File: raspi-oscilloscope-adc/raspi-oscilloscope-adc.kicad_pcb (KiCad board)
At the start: 2 copper layers, 80 x 47.5 mm, 26 parts, among them J1 Conn_Coaxial, J2 Conn_01x10_Male, J3 Conn_01x02_Male, SW1 SR10010F-0106-20F0B-C7-N-0027, U1 ECS-220B-100, U2 TLC5510INSR, U3 OPA690, U4 SN74LS245N

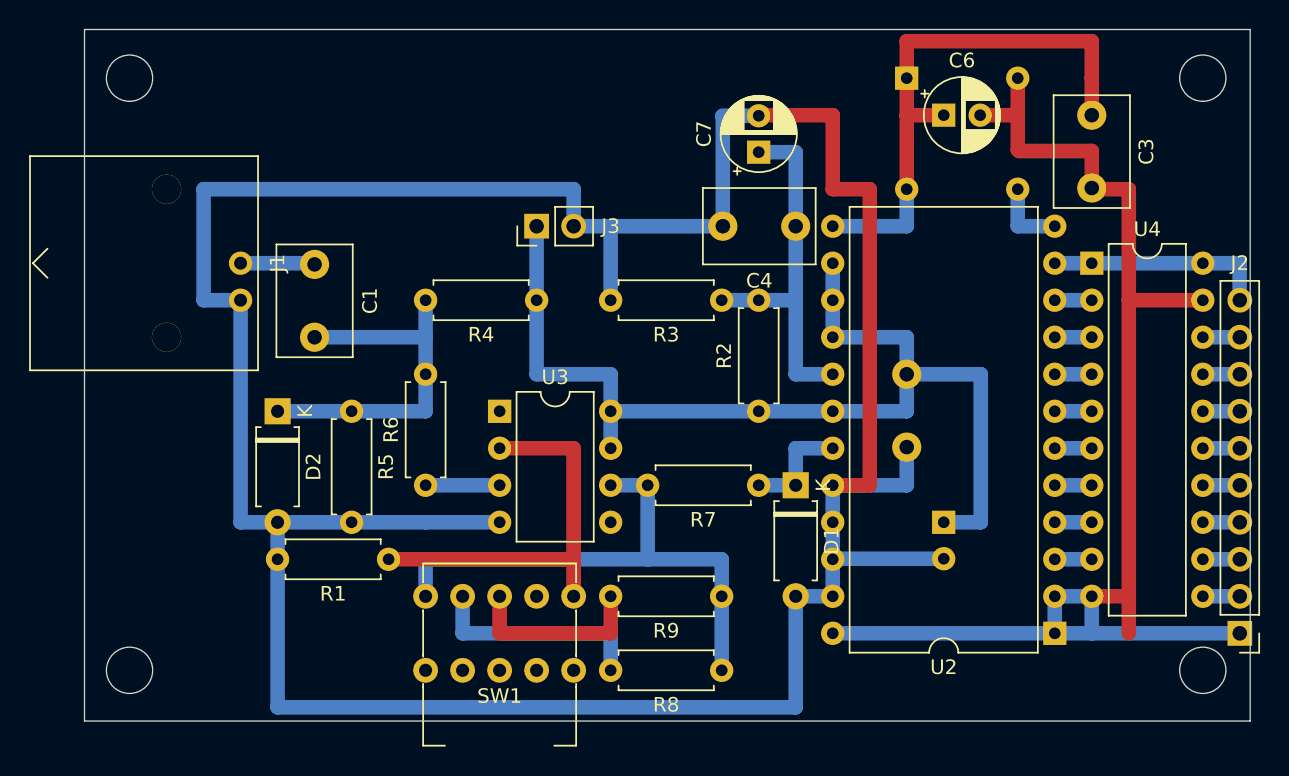
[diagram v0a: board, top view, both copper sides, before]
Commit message: Fix error in board
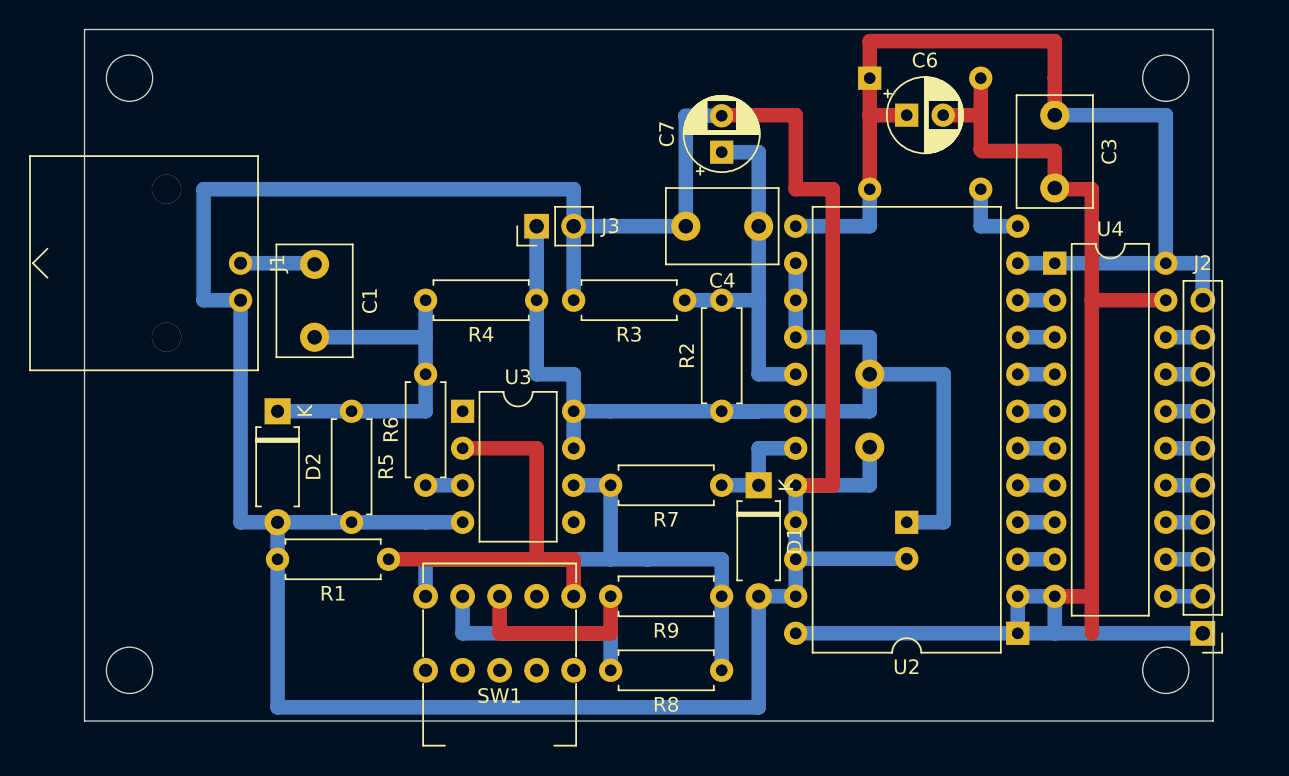
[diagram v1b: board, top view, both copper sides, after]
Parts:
- moved R3 2.54 mm to (147.3, 88.9)
- moved C2 2.54 mm to (160.0, 94.0)
- moved C3 2.54 mm to (172.7, 76.2)
- moved C4 2.54 mm to (152.4, 83.8)
- moved C5 2.54 mm to (162.6, 104.1)
- moved C6 2.54 mm to (162.6, 76.2)
- moved C7 2.54 mm to (149.9, 78.7)
- moved D1 2.54 mm to (152.4, 101.6)
- moved J2 2.54 mm to (182.9, 111.8)
- moved R2 2.54 mm to (149.9, 96.5)
- moved R7 2.54 mm to (149.9, 101.6)
- moved U1 2.54 mm to (160.0, 73.7)
- moved U2 2.54 mm to (170.2, 111.8)
- moved U3 2.54 mm to (132.1, 96.5)
- moved U4 2.54 mm to (172.7, 86.4)
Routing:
- net +5VD: track 53.3 -> 71.1 mm
- net GNDA: track 213.4 -> 205.8 mm
- net Net-(R6-Pad1): track 5.08 -> 2.54 mm
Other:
- board size 80 x 47.5 mm -> 77.5 x 47.5 mm
